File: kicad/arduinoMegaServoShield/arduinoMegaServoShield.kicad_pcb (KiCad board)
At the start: 2 copper layers, 85.1 x 53.3 mm, 32 parts, among them J1 Screw_Terminal_01x02, M1 Motor_Servo, M10 Motor_Servo, M11 Motor_Servo, M12 Motor_Servo, M13 Motor_Servo, M14 Motor_Servo, M15 Motor_Servo, M16 Motor_Servo, M17 Motor_Servo, M18 Motor_Servo, M19 Motor_Servo, M2 Motor_Servo, M20 Motor_Servo, M21 Motor_Servo, M22 Motor_Servo, M23 Motor_Servo, M24 Motor_Servo, M25 Motor_Servo, M26 Motor_Servo, M27 Motor_Servo, M28 Motor_Servo, M29 Motor_Servo, M3 Motor_Servo, M4 Motor_Servo, M5 Motor_Servo, M6 Motor_Servo, M7 Motor_Servo, M8 Motor_Servo, M9 Motor_Servo

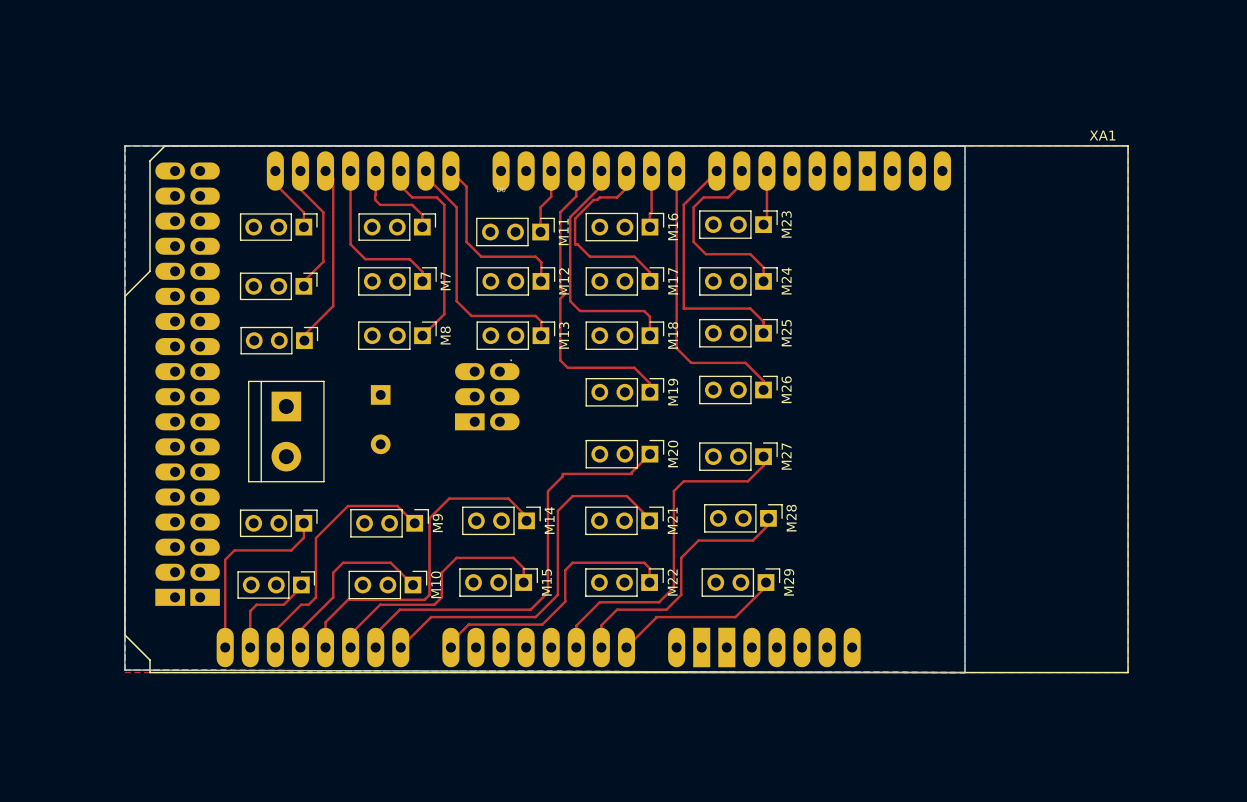
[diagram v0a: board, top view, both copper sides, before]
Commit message: improved layout
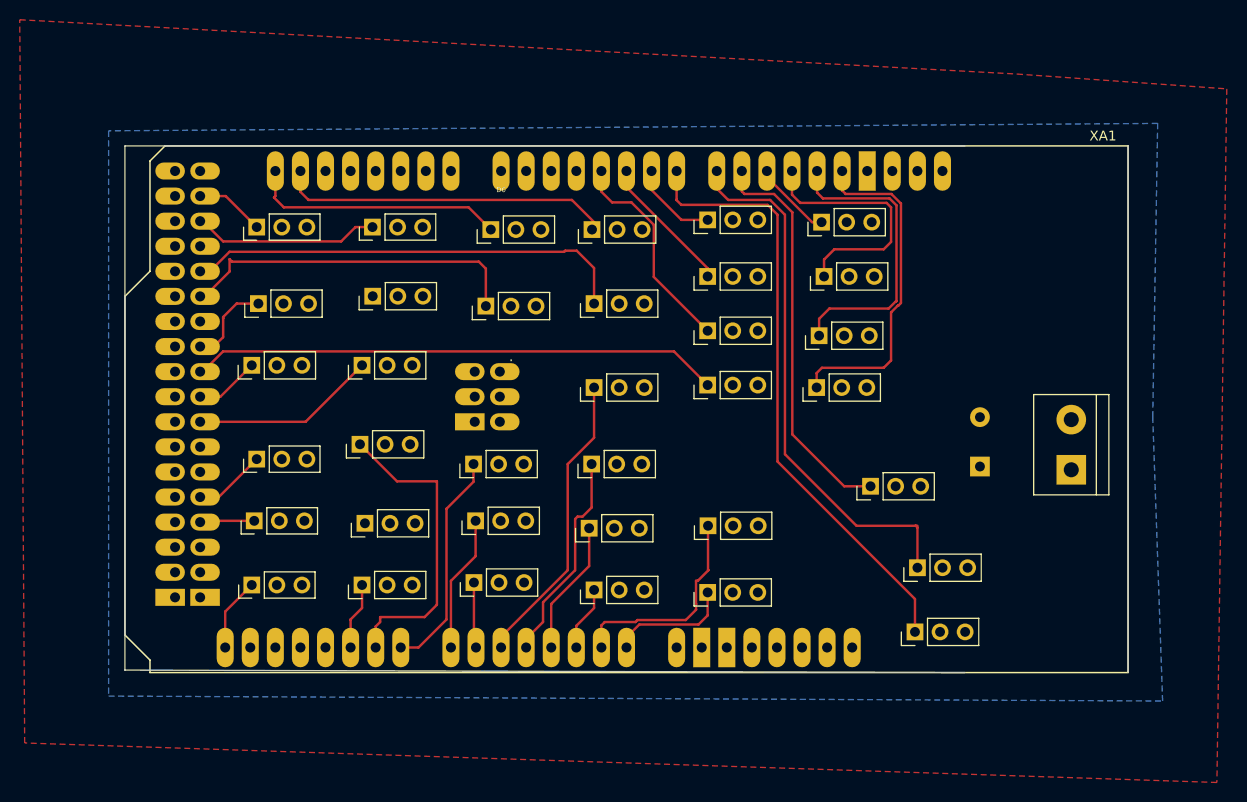
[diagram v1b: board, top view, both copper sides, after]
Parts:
- removed M22, M24, M3: Motor_Servo, Connector_PinHeader_2.54mm:PinHeader_1x03_P2.54mm_Vertical
- added M30: Motor_Servo, Connector_PinHeader_2.54mm:PinHeader_1x03_P2.54mm_Vertical, F.Cu at (38.9, 33.8)
- added M31: Motor_Servo, Connector_PinHeader_2.54mm:PinHeader_1x03_P2.54mm_Vertical, F.Cu at (38.2, 40.0)
- added M34: Motor_Servo, Connector_PinHeader_2.54mm:PinHeader_1x03_P2.54mm_Vertical, F.Cu at (60.7, 50.0)
- added M35: Motor_Servo, Connector_PinHeader_2.54mm:PinHeader_1x03_P2.54mm_Vertical, F.Cu at (105.4, 67.0)
- added M36: Motor_Servo, Connector_PinHeader_2.54mm:PinHeader_1x03_P2.54mm_Vertical, F.Cu at (105.7, 60.5)
- added M37: Motor_Servo, Connector_PinHeader_2.54mm:PinHeader_1x03_P2.54mm_Vertical, F.Cu at (95.5, 42.2)
- added M38: Motor_Servo, Connector_PinHeader_2.54mm:PinHeader_1x03_P2.54mm_Vertical, F.Cu at (95.7, 37.0)
- added M39: Motor_Servo, Connector_PinHeader_2.54mm:PinHeader_1x03_P2.54mm_Vertical, F.Cu at (96.2, 31.0)
- added M40: Motor_Servo, Connector_PinHeader_2.54mm:PinHeader_1x03_P2.54mm_Vertical, F.Cu at (96.0, 25.5)
- added M41: Motor_Servo, Connector_PinHeader_2.54mm:PinHeader_1x03_P2.54mm_Vertical, F.Cu at (100.9, 52.2)
- moved J1 79.8 mm to (121.2, 50.6), turned to 90 degrees
- moved C3 61.1 mm to (112.0, 50.2), turned to 90 degrees
- moved M23 23.8 mm to (72.9, 42.2), turned to 90 degrees
- moved M26 23.8 mm to (72.7, 26.2), turned to 90 degrees
- moved M27 21.8 mm to (72.9, 62.8), turned to 90 degrees
- moved M13 21.4 mm to (49.2, 48.0), turned to 90 degrees
- moved M29 21.4 mm to (72.7, 50.0), turned to 90 degrees
- moved M19 18.4 mm to (84.4, 25.3), turned to 90 degrees
- moved M28 18.2 mm to (72.4, 56.5), turned to 90 degrees
- moved M2 18.1 mm to (38.8, 49.5), turned to 90 degrees
- moved M14 17.9 mm to (49.4, 62.2), turned to 90 degrees
- moved M25 17.4 mm to (72.9, 33.8), turned to 90 degrees
- moved M15 17.2 mm to (49.7, 56.0), turned to 90 degrees
- moved M16 17.0 mm to (84.4, 42.0), turned to 90 degrees
- moved M20 15.2 mm to (84.4, 63.0), turned to 90 degrees
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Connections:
- M1 pad 2: +5VP -> unconnected-(M1-+-Pad2)
- M1 pad 3: GND -> unconnected-(M1---Pad3)
- M11 pad 2: +5VP -> unconnected-(M11-+-Pad2)
- M11 pad 3: GND -> unconnected-(M11---Pad3)
- M12 pad 2: +5VP -> unconnected-(M12-+-Pad2)
- M12 pad 3: GND -> unconnected-(M12---Pad3)
- M13 pad 2: +5VP -> unconnected-(M13-+-Pad2)
- M13 pad 3: GND -> unconnected-(M13---Pad3)
- M15 pad 1: Net-(M15-PWM) -> unconnected-(M15-PWM-Pad1)
- M16 pad 2: +5VP -> unconnected-(M16-+-Pad2)
- M16 pad 3: GND -> unconnected-(M16---Pad3)
- M17 pad 2: +5VP -> unconnected-(M17-+-Pad2)
- M17 pad 3: GND -> unconnected-(M17---Pad3)
- M18 pad 2: +5VP -> unconnected-(M18-+-Pad2)
- M18 pad 3: GND -> unconnected-(M18---Pad3)
- M19 pad 3: GND -> unconnected-(M19---Pad3)
- M23 pad 2: +5VP -> unconnected-(M23-+-Pad2)
- M23 pad 3: GND -> unconnected-(M23---Pad3)
- M25 pad 2: +5VP -> unconnected-(M25-+-Pad2)
- M25 pad 3: GND -> unconnected-(M25---Pad3)
- M26 pad 2: +5VP -> unconnected-(M26-+-Pad2)
- M26 pad 3: GND -> unconnected-(M26---Pad3)
- M27 pad 2: +5VP -> unconnected-(M27-+-Pad2)
- M27 pad 3: GND -> unconnected-(M27---Pad3)
- M28 pad 2: +5VP -> unconnected-(M28-+-Pad2)
- M28 pad 3: GND -> unconnected-(M28---Pad3)
- M29 pad 2: +5VP -> unconnected-(M29-+-Pad2)
- M29 pad 3: GND -> unconnected-(M29---Pad3)
- M4 pad 2: unconnected-(M4-+-Pad2) -> +5VP
- M4 pad 3: unconnected-(M4---Pad3) -> GND
- M6 pad 2: +5VP -> unconnected-(M6-+-Pad2)
- M6 pad 3: GND -> unconnected-(M6---Pad3)
- M7 pad 2: +5VP -> unconnected-(M7-+-Pad2)
- M7 pad 3: GND -> unconnected-(M7---Pad3)
- M8 pad 2: +5VP -> unconnected-(M8-+-Pad2)
- M8 pad 3: GND -> unconnected-(M8---Pad3)
- XA1 pad A0: Net-(M29-PWM) -> Net-(M20-PWM)
- XA1 pad A1: Net-(M28-PWM) -> Net-(M21-PWM)
- XA1 pad A10: Net-(M15-PWM) -> Net-(M14-PWM)
- XA1 pad A11: Net-(M14-PWM) -> unconnected-(XA1-PadA11)
- XA1 pad A12: Net-(M10-PWM) -> unconnected-(XA1-PadA12)
- XA1 pad A13: Net-(M9-PWM) -> unconnected-(XA1-PadA13)
- XA1 pad A14: Net-(M5-PWM) -> unconnected-(XA1-PadA14)
- XA1 pad A15: Net-(M4-PWM) -> Net-(M5-PWM)
- XA1 pad A3: unconnected-(XA1-PadA3) -> Net-(M28-PWM)
- XA1 pad A4: unconnected-(XA1-PadA4) -> Net-(M29-PWM)
- XA1 pad A5: unconnected-(XA1-PadA5) -> Net-(M23-PWM)
- XA1 pad A6: unconnected-(XA1-PadA6) -> Net-(M9-PWM)
- XA1 pad A7: Net-(M22-PWM) -> Net-(M10-PWM)
- XA1 pad A8: Net-(M21-PWM) -> Net-(M34-PWM)
- XA1 pad A9: Net-(M20-PWM) -> Net-(M13-PWM)
- XA1 pad D10: Net-(M23-PWM) -> Net-(M40-PWM)
- XA1 pad D11: unconnected-(XA1-PadD11) -> Net-(M39-PWM)
- XA1 pad D12: unconnected-(XA1-PadD12) -> Net-(M38-PWM)
- XA1 pad D13: unconnected-(XA1-PadD13) -> Net-(M37-PWM)
- XA1 pad D14: Net-(M12-PWM) -> unconnected-(XA1-D14/TX3-PadD14)
- XA1 pad D15: Net-(M13-PWM) -> unconnected-(XA1-D15/RX3-PadD15)
- XA1 pad D16: Net-(M8-PWM) -> unconnected-(XA1-D16/TX2-PadD16)
- XA1 pad D17: Net-(M6-PWM) -> unconnected-(XA1-D17/RX2-PadD17)
- XA1 pad D18: Net-(M7-PWM) -> unconnected-(XA1-D18/TX1-PadD18)
- XA1 pad D19: Net-(M3-PWM) -> unconnected-(XA1-D19/RX1-PadD19)
- XA1 pad D2: Net-(M11-PWM) -> unconnected-(XA1-D2_INT0-PadD2)
- XA1 pad D20: Net-(M2-PWM) -> Net-(M26-PWM)
- XA1 pad D21: Net-(M1-PWM) -> Net-(M11-PWM)
- XA1 pad D22: unconnected-(XA1-PadD22) -> Net-(M1-PWM)
- XA1 pad D24: unconnected-(XA1-PadD24) -> Net-(M6-PWM)
- XA1 pad D28: unconnected-(XA1-PadD28) -> Net-(M25-PWM)
- XA1 pad D3: Net-(M19-PWM) -> unconnected-(XA1-D3_INT1-PadD3)
- XA1 pad D30: unconnected-(XA1-PadD30) -> Net-(M12-PWM)
- XA1 pad D32: unconnected-(XA1-PadD32) -> Net-(M7-PWM)
- XA1 pad D34: unconnected-(XA1-PadD34) -> Net-(M30-PWM)
- XA1 pad D36: unconnected-(XA1-PadD36) -> Net-(M16-PWM)
- XA1 pad D38: unconnected-(XA1-PadD38) -> Net-(M31-PWM)
- XA1 pad D4: Net-(M18-PWM) -> Net-(M17-PWM)
- XA1 pad D40: unconnected-(XA1-PadD40) -> Net-(M8-PWM)
- XA1 pad D46: unconnected-(XA1-PadD46) -> Net-(M2-PWM)
- XA1 pad D48: unconnected-(XA1-PadD48) -> Net-(M4-PWM)
- XA1 pad D5: Net-(M17-PWM) -> Net-(M18-PWM)
- XA1 pad D6: Net-(M16-PWM) -> Net-(M19-PWM)
- XA1 pad D7: Net-(M26-PWM) -> Net-(M35-PWM)
- XA1 pad D8: Net-(M25-PWM) -> Net-(M36-PWM)
- XA1 pad GND4: GND -> unconnected-(XA1-SPI_GND-PadGND4)
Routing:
- net Net-(M35-PWM): track 0.00 -> 61.8 mm
- net Net-(M36-PWM): track 0.00 -> 53.0 mm
- net Net-(M16-PWM): track 5.92 -> 53.4 mm
- net Net-(M37-PWM): track 0.00 -> 34.3 mm
- net Net-(M20-PWM): track 42.9 -> 11.5 mm
- net Net-(M38-PWM): track 0.00 -> 30.8 mm
- net Net-(M27-PWM): track 34.5 -> 6.58 mm
- net Net-(M22-PWM): track 27.5 -> 0.00 mm
- net Net-(M14-PWM): track 33.8 -> 6.82 mm
- net Net-(M39-PWM): track 0.00 -> 25.7 mm
- net Net-(M15-PWM): track 25.4 -> 0.00 mm
- net Net-(M23-PWM): track 5.57 -> 29.2 mm
- net Net-(M34-PWM): track 0.00 -> 22.7 mm
- net Net-(M19-PWM): track 31.2 -> 8.86 mm
- net Net-(M41-PWM): track 20.2 -> 40.7 mm
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- removed copper zone on B.Cu, net (none)
- removed copper zone on B.Cu, net unconnected-(XA1-3.3V-Pad3V3)
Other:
- board size 85.1 x 53.3 mm -> 101.6 x 53.4 mm
